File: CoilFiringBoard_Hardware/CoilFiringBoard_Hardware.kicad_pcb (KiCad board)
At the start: 2 copper layers, 101.6 x 76.2 mm, 20 parts, among them Q1 Q_NMOS_GDS, Q2 Q_NMOS_GDS

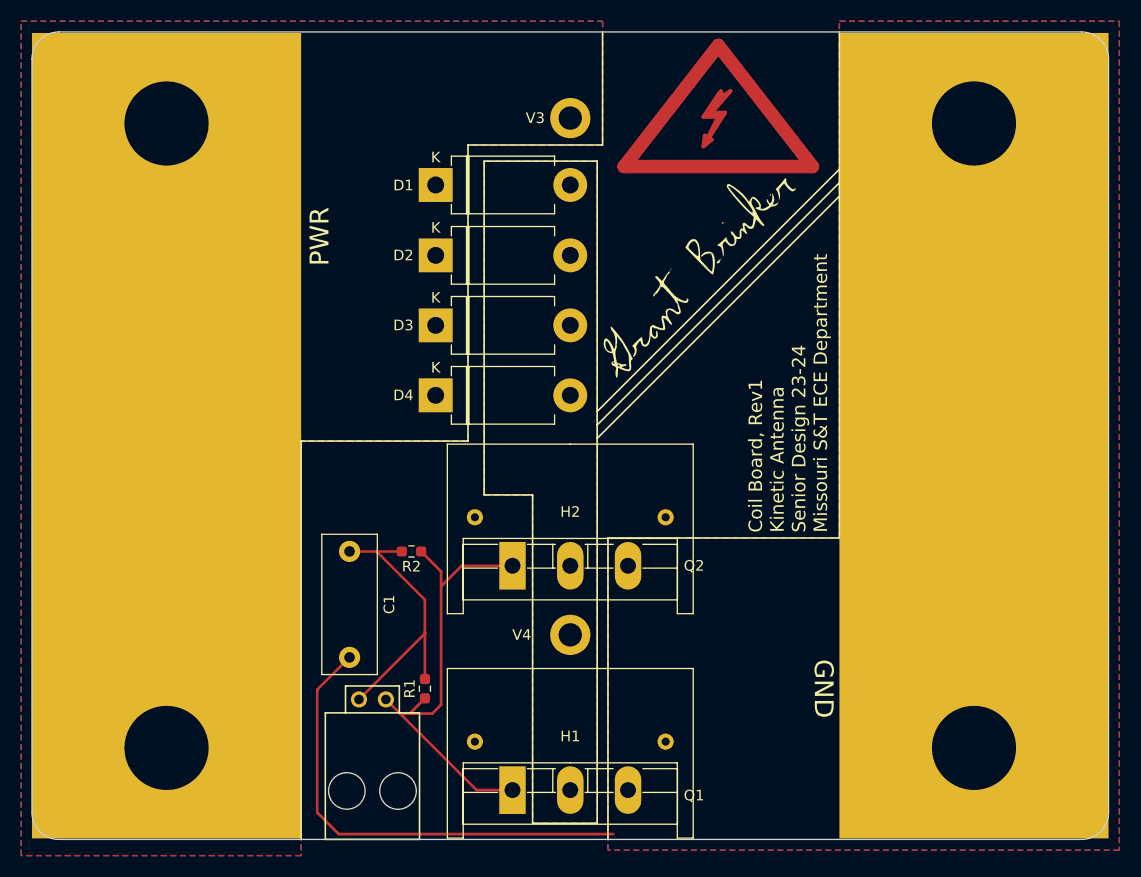
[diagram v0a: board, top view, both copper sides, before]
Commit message: Made most review changes
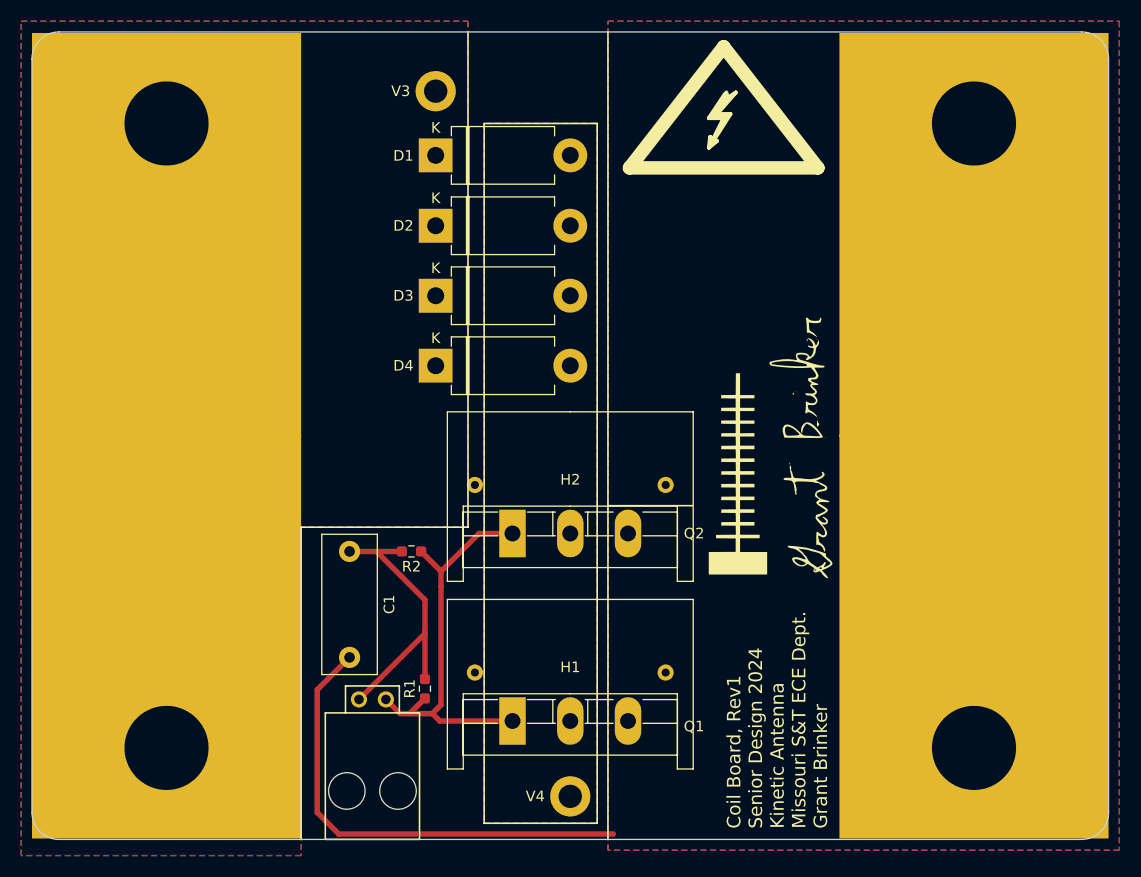
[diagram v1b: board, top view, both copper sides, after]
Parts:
- added G***: LOGO, MRDT_Silkscreens:yagi, F.Cu at (130.0, 80.3)
- moved G*** 20.0 mm to (136.1, 77.7), turned to 90 degrees
- moved V4 15.2 mm to (114.3, 110.7)
- moved V3 13.0 mm to (101.6, 44.2)
- moved H1 6.52 mm to (114.3, 99.1)
- moved Q1 6.52 mm to (108.8, 103.6)
- moved H2 3.05 mm to (114.3, 81.4)
- moved Q2 3.05 mm to (108.8, 85.9)
- moved D1 2.79 mm to (101.6, 50.3)
- moved D2 2.79 mm to (101.6, 56.9)
- moved D3 2.79 mm to (101.6, 63.5)
- moved D4 2.79 mm to (101.6, 70.1)
- moved REF** 0.52 mm to (128.8, 47.6)
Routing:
- net Net-(Q1-G): track 44.5 -> 39.5 mm
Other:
- board text added: "Coil Board, Rev1 Senior Design 2024 Kinetic Antenna Missouri S&T ECE Dept. Grant Brinker"
- board text removed: "Coil Board, Rev1 Kinetic Antenna Senior Design 23-24 Missouri S&T ECE Department"
- board text removed: "GND"
- board text removed: "PWR"
